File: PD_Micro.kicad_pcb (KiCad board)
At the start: 2 copper layers, 72.6 x 53.7 mm, 43 parts, among them J3 Conn_01x02, Q1 DMP3017SFK, Q2 DTC143E, SW1 SW_DPST_x2, SW2 SW_Push, SW4 SW_DPST_x2, SW5 SW_DIP_x06, SW6 SW_Push, U1 TPS62175DQC, U2 SRV05-4, U3 Pico, U4 FUSB302BMPX, U5 ACS723xMATR-10AB, U6 oledSym

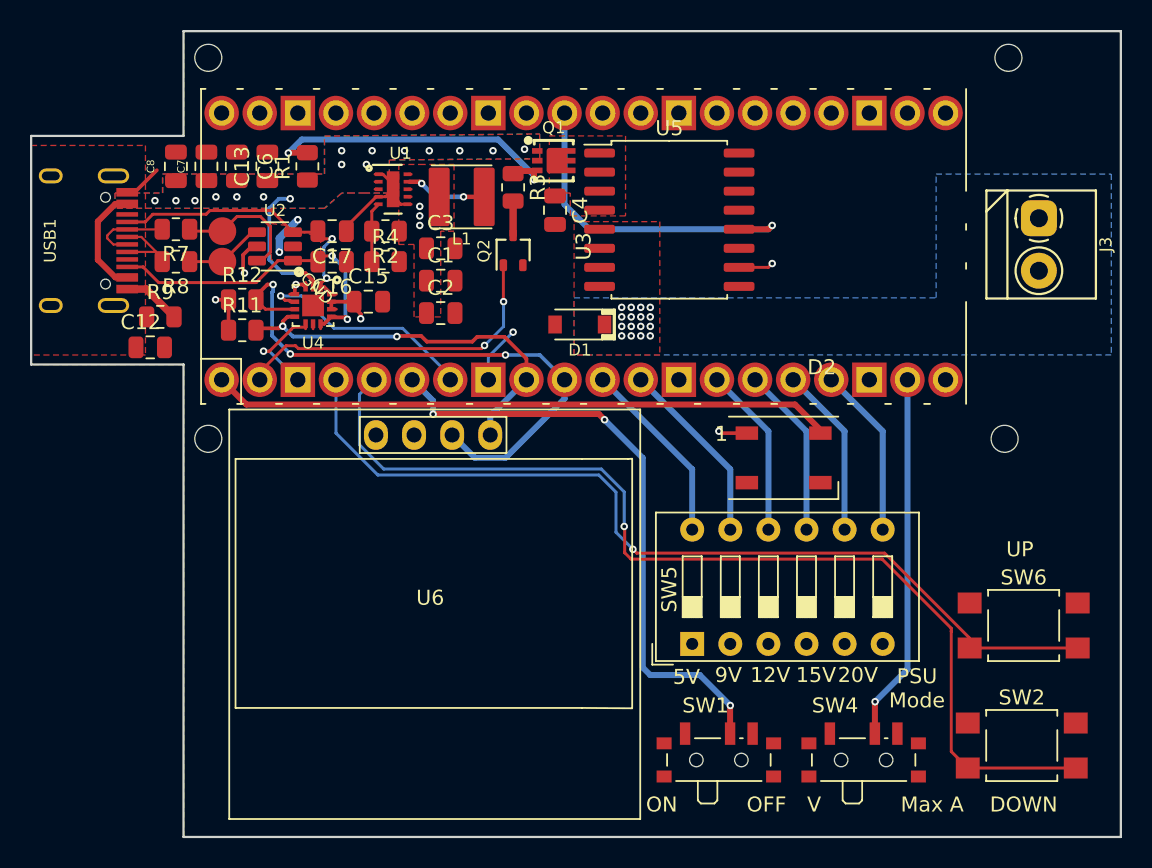
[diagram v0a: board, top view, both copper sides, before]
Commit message: differential-pair
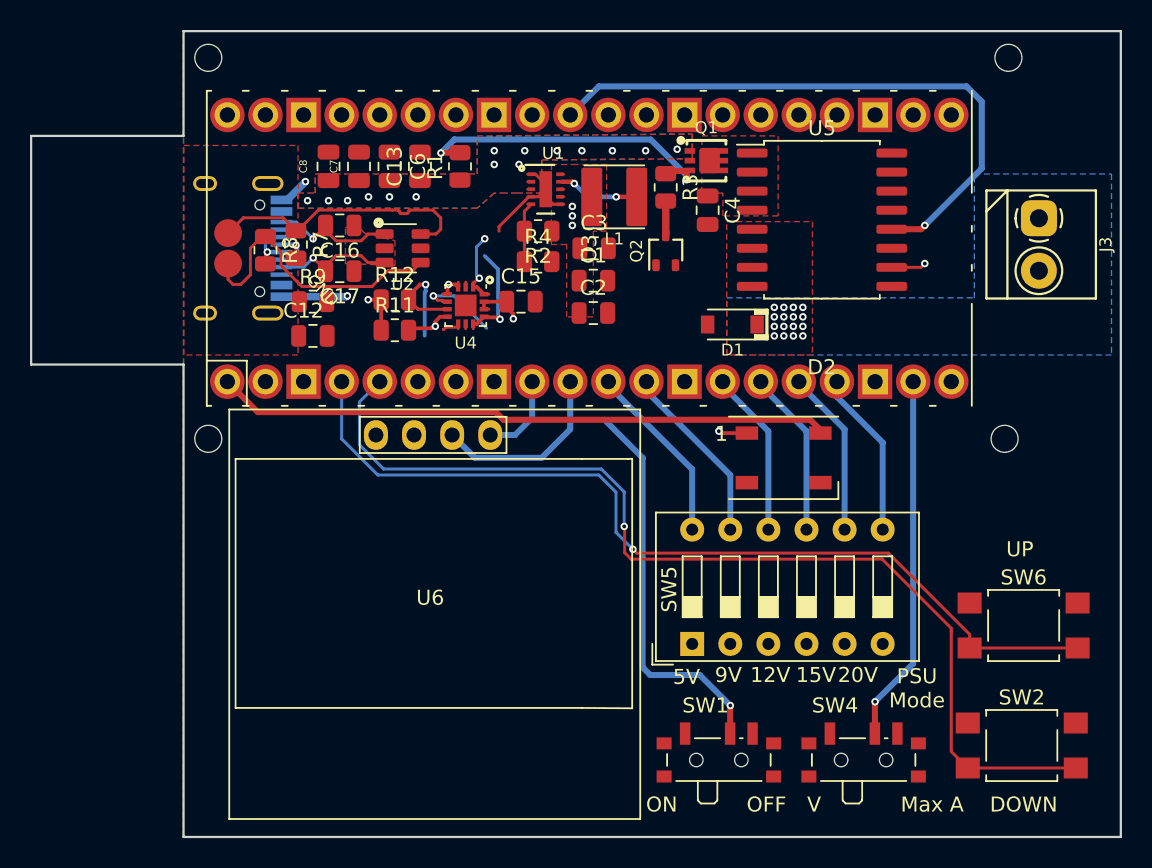
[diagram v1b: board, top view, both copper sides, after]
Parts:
- USB1: moved to B.Cu
- moved C12 10.9 mm to (183.6, 107.1)
- moved USB1 10.3 mm to (173.9, 101.3), turned to 90 degrees
- moved C3 10.2 mm to (202.4, 101.3)
- moved R9 10.2 mm to (183.6, 104.8)
- moved C1 10.2 mm to (202.3, 103.4)
- moved C13 10.2 mm to (190.8, 95.8)
- moved C15 10.2 mm to (197.5, 104.8)
- moved C2 10.2 mm to (202.3, 105.6)
- moved C4 10.2 mm to (210.0, 98.7)
- moved C6 10.2 mm to (188.7, 95.8)
- moved C7 10.2 mm to (186.7, 95.8)
- moved C8 10.2 mm to (184.7, 95.8)
- moved D1 10.2 mm to (211.6, 106.3)
- moved L1 10.2 mm to (203.7, 97.8)
- moved Q1 10.2 mm to (209.9, 95.4)
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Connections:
- net /DN renamed /D_N
- net /DP renamed /D_P
- net Net-(R7-Pad1) renamed /D1_N
- net Net-(R8-Pad1) renamed /D1_P
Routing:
- net ENOUT: track 22.3 -> 0.51 mm, vias 2 -> 0
- net SCL: track 39.5 -> 20.2 mm, vias 3 -> 1
- net SDA: track 27.0 -> 8.78 mm, vias 2 -> 1
- net ADC0: track 23.0 -> 40.8 mm
- net VBUS: track 16.5 -> 0.00 mm, vias 17 -> 15
- net Net-(SW1-Pad2): track 40.8 -> 26.3 mm, vias 3 -> 1
- net /D1_P: track 5.41 -> 19.0 mm
- net GND: track 27.1 -> 15.1 mm, vias 4 -> 2
- net INT_N: track 14.6 -> 5.32 mm
- net /D1_N: track 9.01 -> 18.2 mm
- net /CC1: track 19.1 -> 12.7 mm, vias 2 -> 3
- net /CC2: track 21.6 -> 15.2 mm
- net +5V: track 13.9 -> 11.5 mm, vias 9 -> 8
- net /D_N: track 5.95 -> 3.90 mm, vias 0 -> 1
- net /D_P: track 3.54 -> 3.84 mm, vias 0 -> 1
